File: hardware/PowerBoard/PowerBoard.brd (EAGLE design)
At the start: 90 x 56 mm, 136 parts, among them J1 CON-HRS-DM3AT, J2 CON-ZX62R-B-5P, J3 CON-FTSH-105-01-L-DV-K, J4 CON-S2B-PH-SM4-TB, J5 CON-PJ-102A, J6 CON-71741-0002-TOP, J7 SWITCH-CJS-1200-1200, M1 MOUNT-HOLE3.3, M2 MOUNT-HOLE3.3, M3 MOUNT-HOLE3.3, M4 MOUNT-HOLE3.3, M5 FIDUCIAL1X2, M6 FIDUCIAL1X2, M7 FIDUCIAL1X2, M8 FIDUCIAL1X2, Q1 SI2323CDS, Q2 SI2312CDS, Q3 SI2333CDS, Q4 SI2333CDS, SW1 SWITCH-SPST, SW2 SWITCH-MS12ASG30, SW3 SWITCH-ESWITCH-TL3340G, U1 LTC4361-2DC, U10 MAX9938FEUK, U11 MAX9938FEUK, U12 MAX9938FEUK, U13 STM32F10XCXT6, U14 LTC2942-1, U15 USBLC6-2, U2 LTC4085, U3 XC6220B331MR-G, U4 XC6220B331MR-G, U5 XC9236A15DMR-G, U6 MIC94043, U8 MAX9938FEUK, U9 MAX9938FEUK, X1 ECX-2236, X2 ECX-31B

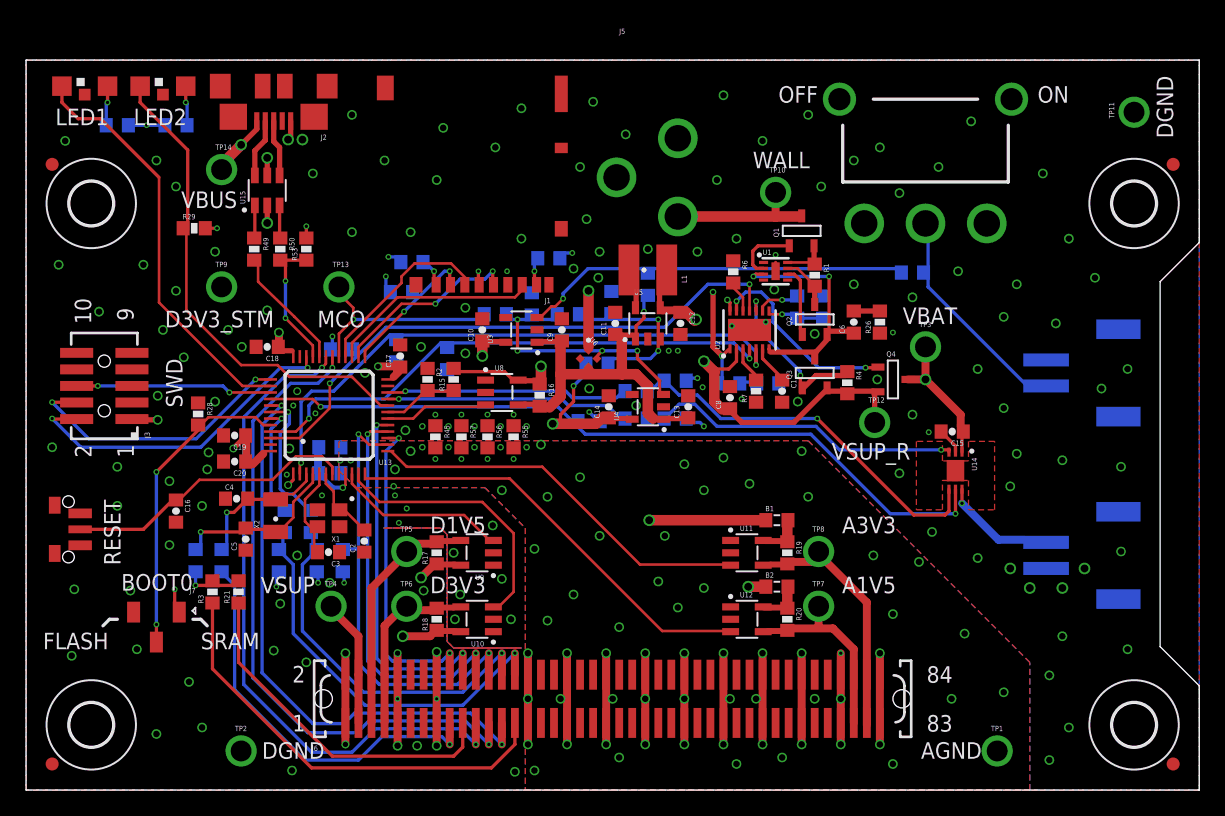
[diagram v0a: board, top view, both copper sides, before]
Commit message: - Air wires eliminated
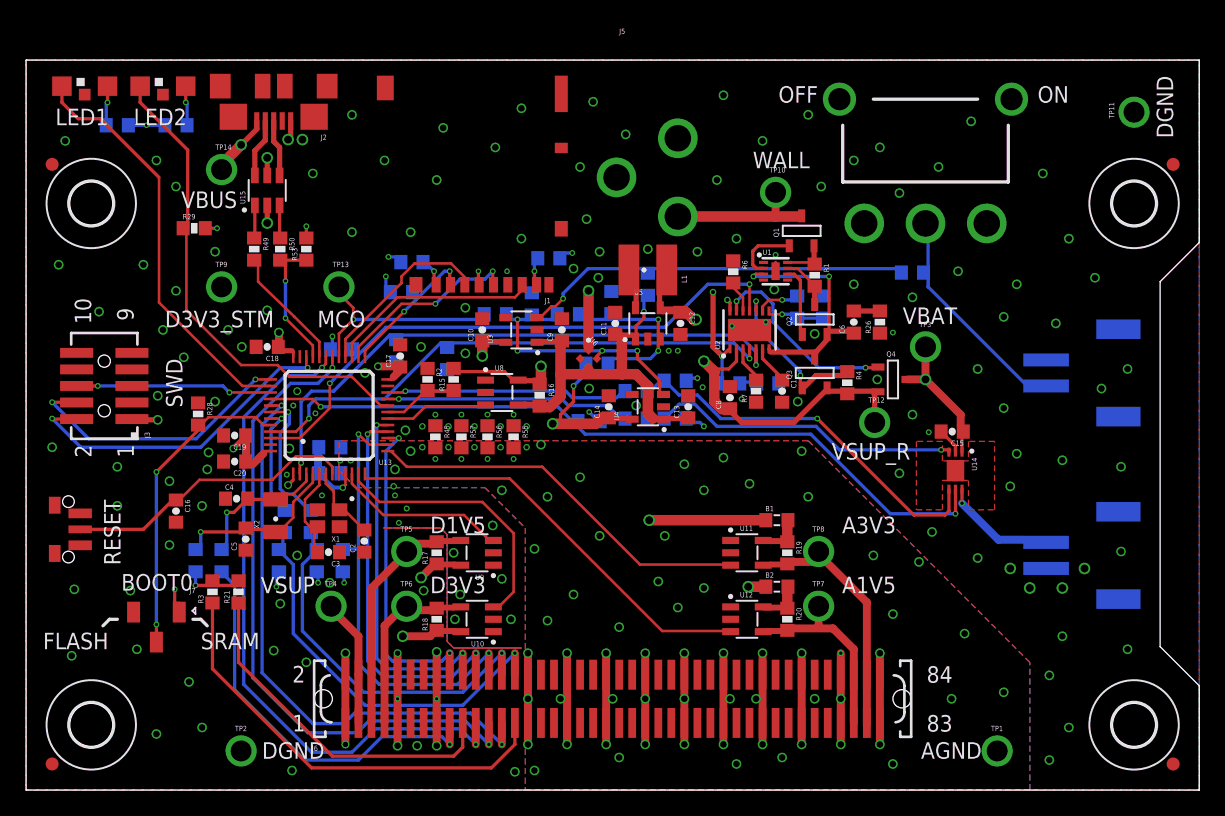
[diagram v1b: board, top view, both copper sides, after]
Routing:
- net D3V3_STM: track 29.9 -> 41.8 mm
- net VSUP_I: track 26.2 -> 33.3 mm
- net VSUP_R: track 39.8 -> 45.0 mm
- net D3V3_I: track 21.0 -> 24.3 mm
- net D3V3: track 15.9 -> 18.8 mm
- net D3V3_STM-EN-SW: track 15.9 -> 18.5 mm
- net D1V5_I: track 9.61 -> 12.2 mm
- net D1V5-EN: track 11.2 -> 13.7 mm
- net D1V5: track 11.8 -> 14.0 mm
- net PC15-S: track 10.5 -> 12.6 mm
- net PA8-EN: track 19.7 -> 21.5 mm
- net VBAT_I: track 7.03 -> 8.77 mm
- net WALL_P: track 17.4 -> 19.0 mm
- net PA8: track 15.4 -> 16.9 mm
- net PC14-S: track 9.30 -> 10.8 mm
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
